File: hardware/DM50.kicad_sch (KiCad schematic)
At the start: 106 parts, among them J1 ST-LINK, J2 USB_C_Receptacle_USB2.0_14P, J3 S2B-PH-K-SLFSN, Q1 MMBT3904, SW1 SW_SPST, SW10 BT_SMD, SW11 BT_SMD, SW12 BT_SMD, SW13 BT_SMD, SW14 BT_SMD, SW15 BT_SMD, SW16 BT_SMD, SW17 BT_SMD, SW18 BT_SMD, SW19 BT_SMD, SW2 BT_SMD, SW20 BT_SMD, SW21 BT_SMD, SW22 BT_SMD, SW23 BT_SMD, SW24 BT_SMD, SW25 BT_SMD, SW26 BT_SMD, SW27 BT_SMD, SW28 BT_SMD, SW29 BT_SMD, SW3 BT_SMD, SW30 BT_SMD, SW31 BT_SMD, SW32 BT_SMD, SW33 BT_SMD, SW34 BT_SMD, SW35 BT_SMD, SW36 BT_SMD, SW37 BT_SMD, SW38 BT_SMD, SW39 BT_SMD, SW4 BT_SMD, SW40 BT_SMD, SW41 BT_SMD, SW42 SW_SPST, SW43 BT_SMD, SW44 BT_SMD, SW45 BT_SMD, SW46 BT_SMD, SW47 BT_SMD, SW48 BT_SMD, SW49 BT_SMD, SW5 BT_SMD, SW50 BT_SMD, SW51 BT_SMD, SW52 BT_SMD, SW6 BT_SMD, SW7 BT_SMD, SW8 BT_SMD, SW9 BT_SMD, U1 EA_DOGL128X-6, U2 STM32U535CBT6, U3 AT25SF641, U4 USBLC6-2SC6, U5 ADP2108AUJ-3.3, U6 MCP73831-2-OT, Y1 32768

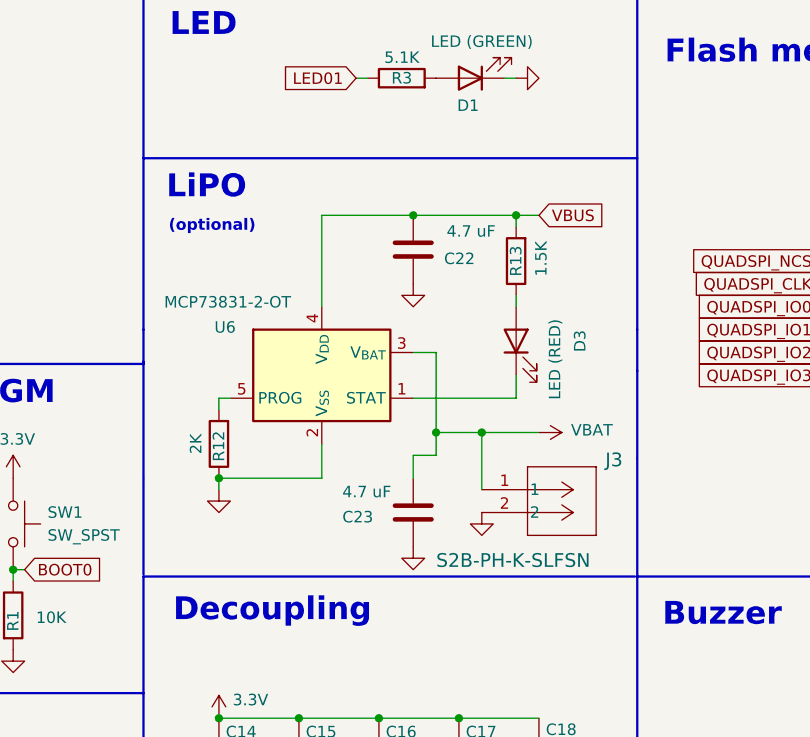
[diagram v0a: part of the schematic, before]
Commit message: pcb changes
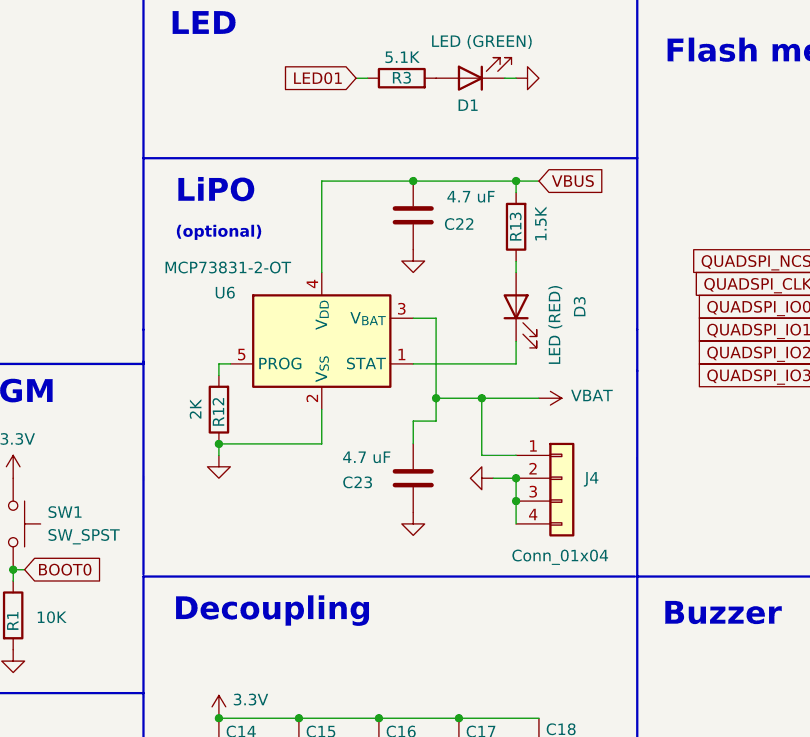
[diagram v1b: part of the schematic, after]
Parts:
- removed J3: S2B-PH-K-SLFSN, DM50:CONN_S2B-PH-K-S_JST, symbol DM50:S2B-PH-K-SLFSN
- added J4: Conn_01x04, DM50:CONN_S2B-ZR-SM4A-TFLFSN_JST, symbol Connector_Generic:Conn_01x04
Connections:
- net GND: now also J4.2 (Pin_2), J4.3 (Pin_3), J4.4 (Pin_4)
- net VBAT: now also J4.1 (Pin_1)
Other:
- moved on the sheet: C22, C23, D3, R12, R13, U6
